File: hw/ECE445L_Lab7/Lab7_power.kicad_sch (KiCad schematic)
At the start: 9 parts, among them J1 JST1.25, J5 ZX62D-B-5PA8_30_, J6 Header2, U5 LP2950-33LPRE3

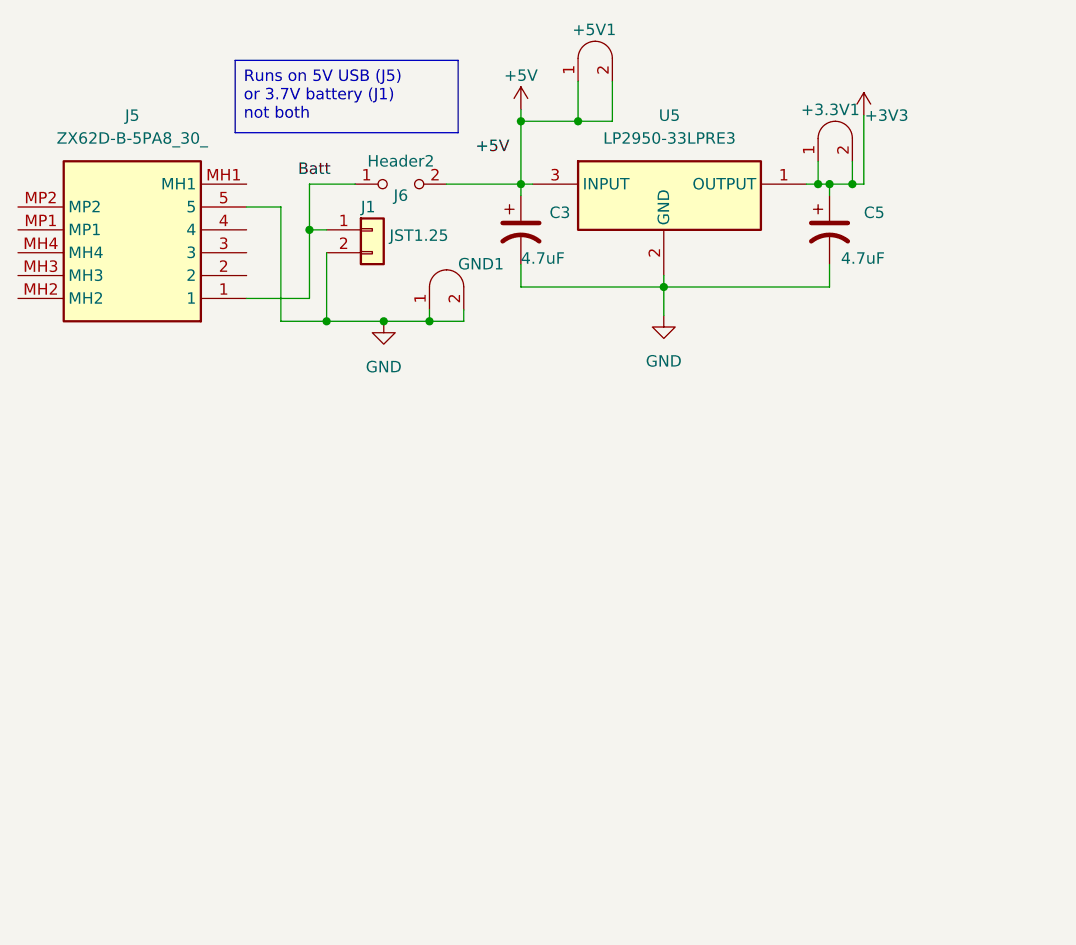
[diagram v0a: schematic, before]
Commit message: mostly finished schem
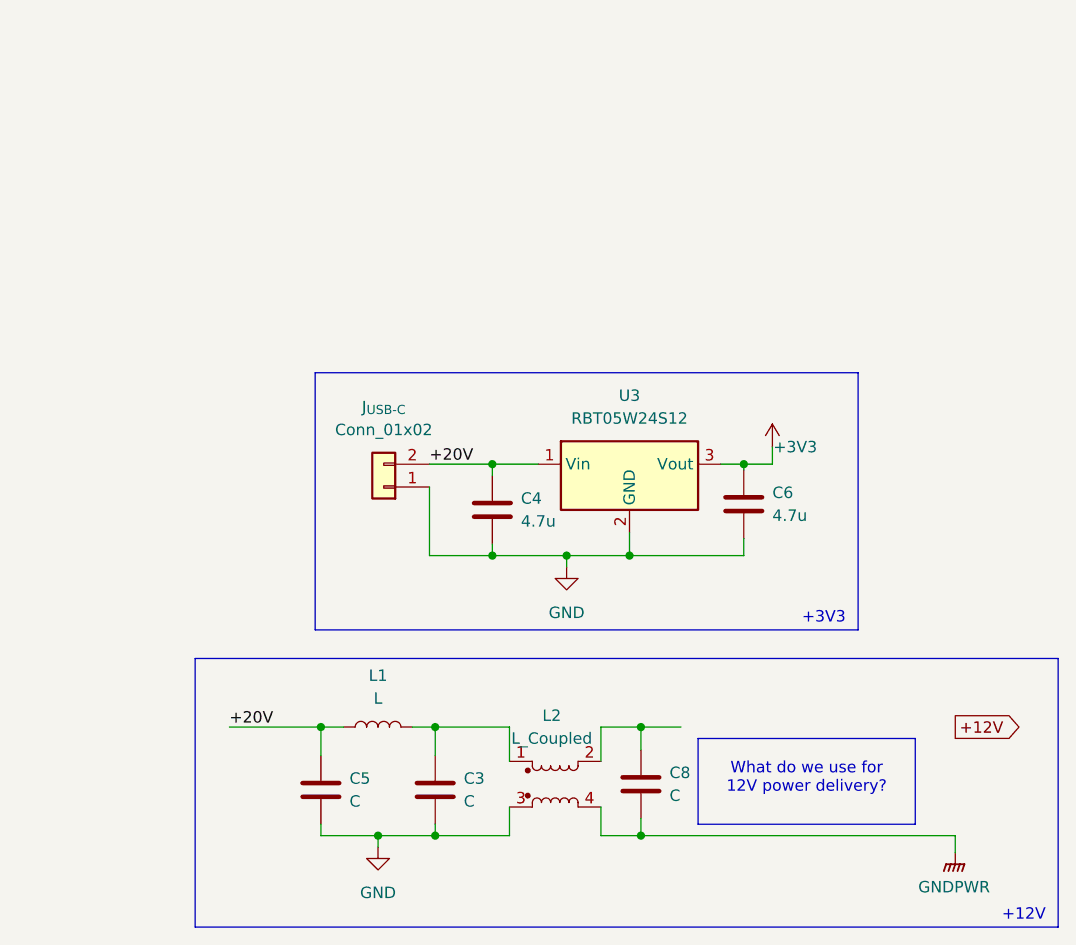
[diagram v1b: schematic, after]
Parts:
- removed +3.3V1: +3.3V, ECE445L:Testpoint_1x02_P2.54mm, symbol ECE445L:Testpoint
- removed +5V1: +5V, ECE445L:Testpoint_1x02_P2.54mm, symbol ECE445L:Testpoint
- removed C3, C5: 4.7uF, ECE445L:CP_Radial_Tantal200mil, symbol ECE445L:C_Polarized
- removed GND1: GND, ECE445L:Testpoint_1x02_P2.54mm, symbol ECE445L:Testpoint
- removed J1: JST1.25, ECE445L:JST-1x02_1.25mm, symbol ECE445L:JST1.25
- removed J5: ZX62D-B-5PA8_30_, ECE445L:ZX62DB5PA830, symbol ECE445L:ZX62D-B-5PA8_30_
- removed J6: Header2, ECE445L:PinHeader_1x02_P2.54mm_Vertical, symbol ECE445L:Header_2
- removed U5: LP2950-33LPRE3, ECE445L:TL431CLPM, symbol ECE445L:LP2950-33LPRE3
- added C3, C5, C8: C, symbol Device:C
- added C4, C6: 4.7u, Capacitor_SMD:C_0805_2012Metric_Pad1.18x1.45mm_HandSolder, symbol Device:C
- added J_{USB-C}: Conn_01x02, symbol Connector_Generic:Conn_01x02
- added L1: L, symbol Device:L
- added L2: L_Coupled, symbol Device:L_Coupled
- added U3: RBT05W24S12, Converter_DCDC:Converter_DCDC_TRACO_TSR0.5-24xx_TSR0.5-24xxx_THT, symbol Converter_DCDC:TSR0.5-2433
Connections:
- net +3V3: now also C6.1, U3.3 (Vout)
- net GND: now also C3.2, C4.2, C5.2, C6.2, J_{USB-C}.1 (Pin_1), L2.3, U3.2 (GND)
- new net: C3.1, L1.2, L2.1
- new net: C8.1, L2.2
- new net +20V: C4.1, C5.1, J_{USB-C}.2 (Pin_2), L1.1, U3.1 (Vin)
- new net GNDPWR: C8.2, L2.4
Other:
- note added: "+12V"
- note added: "+3V3"
- note added: "What do we use for 12V power delivery?"
